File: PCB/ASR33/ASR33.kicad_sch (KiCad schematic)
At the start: 40 parts, among them J2 DC, J3 Power, J4 RUN, J5 Tx, J6 Rx, J7 USB-C-Socket-V, J8 Shelly, Q1 NX7002AK, SW1 SW_Push, U10 ESP32-S3-MINI-1, U2 MD8942, U3 NCR402U, U4 NCR402U, U5 LTV-356T, U7 QR

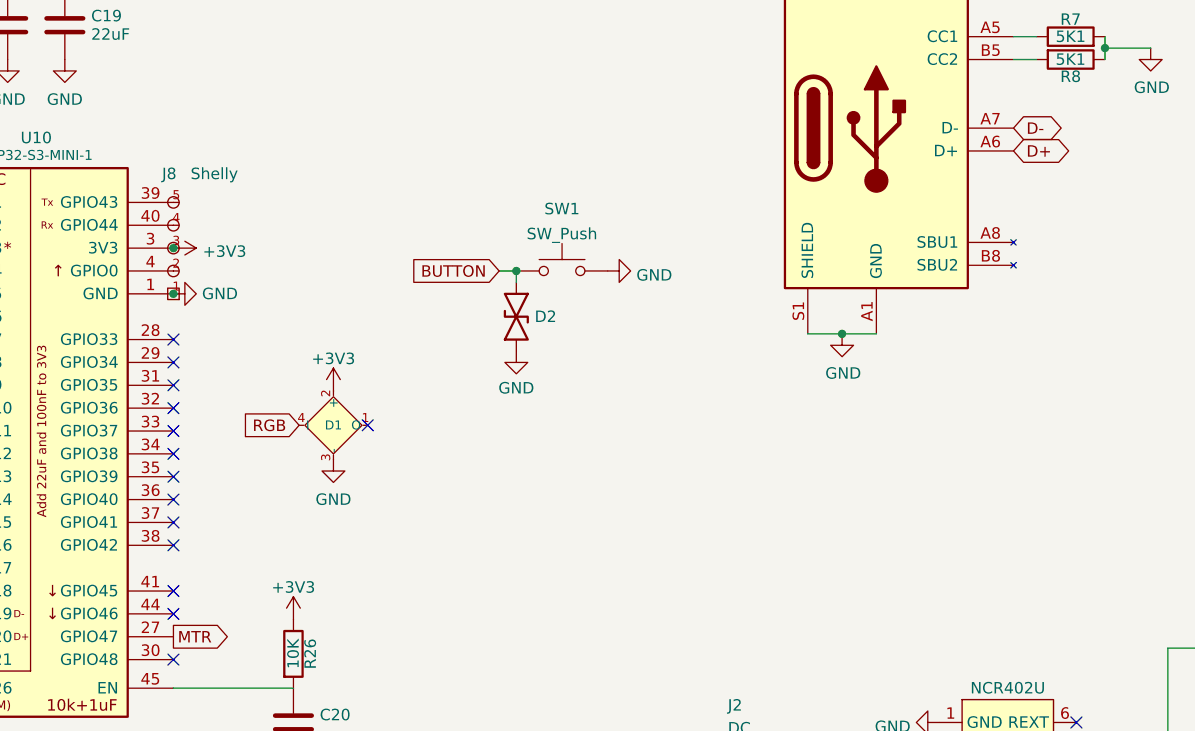
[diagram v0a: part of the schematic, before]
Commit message: Tweaks
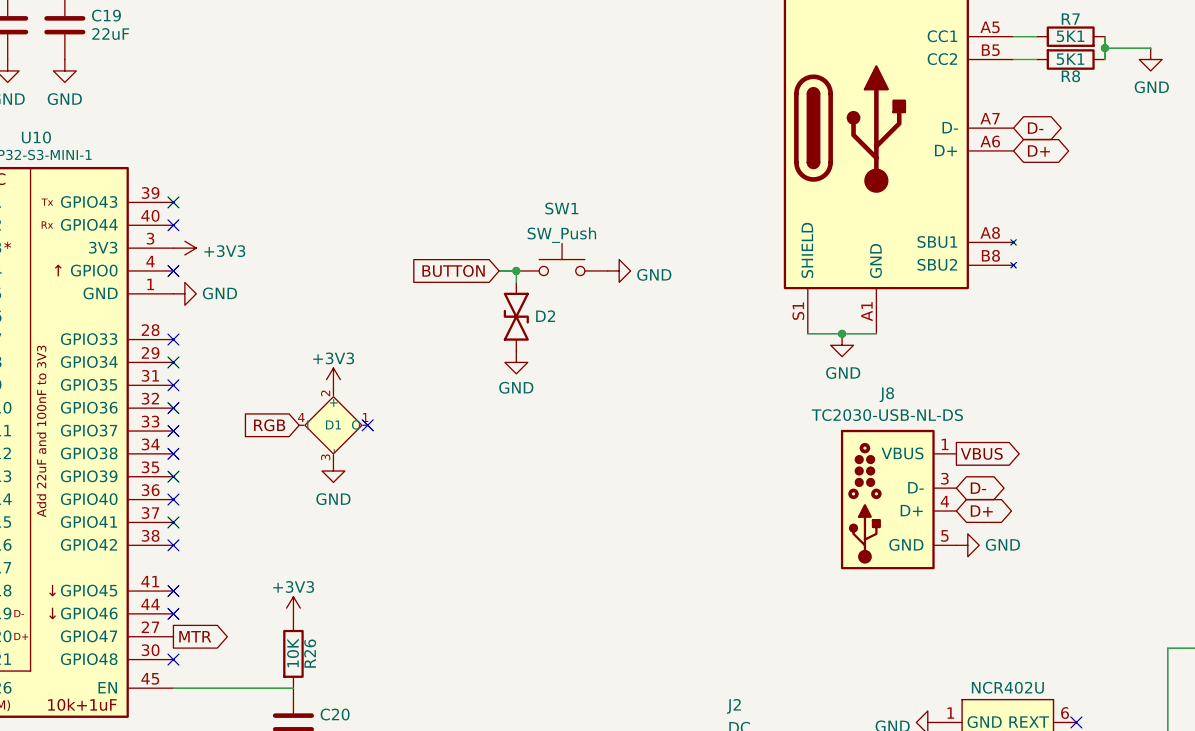
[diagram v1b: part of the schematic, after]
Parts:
- removed J8: Shelly, RevK:Shelly, symbol RevK:Shelly
- added J8: TC2030-USB-NL-DS, RevK:Tag-Connect_TC2030-IDC-NL_2x03_P1.27mm_Vertical, symbol RevK:TC2030-USB-NL
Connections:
- net D+: now also J8.4 (D+)
- net D-: now also J8.3 (D-)
- net GND: now also J8.5 (GND), J8.6 (GND)
- net VBUS: now also J8.1 (VBUS), J8.2 (VBUS)
- no-connect marks 30 -> 33
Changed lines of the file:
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@@
 	)
 	(junction
-		(at 77.47 53.975)
-		(diameter 0)
-		(color 0 0 0 0)
-	)
-	(junction
 		(at 187.96 142.24)
 		(diameter 0)
@@
 	)
 	(junction
-		(at 77.47 59.055)
-		(diameter 0)
-		(color 0 0 0 0)
-	)
-	(junction
 		(at 187.96 111.76)
 		(diameter 0)
@@
 	)
 	(no_connect
+		(at 77.47 48.895)
+	)
+	(no_connect
 		(at 46.99 66.675)
 	)
@@
 	)
 	(no_connect
+		(at 77.47 56.515)
+	)
+	(no_connect
 		(at 46.99 48.895)
 	)
@@
 	)
 	(no_connect
+		(at 77.47 51.435)
+	)
+	(no_connect
 		(at 77.47 81.915)
 	)
@@
 		)
 	)
+	(global_label "D-"
+		(shape bidirectional)
+		(at 164.465 80.645 0)
+		(fields_autoplaced yes)
+		(effects
+			(font
+				(size 1.27 1.27)
+			)
+			(justify left)
+		)
+		(property "Intersheetrefs" "${INTERSHEET_REFS}"
+			(at 170.5909 80.645 0)
+			(effects
+				(font
+					(size 1.27 1.27)
+				)
+				(justify left)
+				(hide yes)
+			)
+		)
+	)
 	(global_label "PWR"
 		(shape input)
@@
 		)
 	)
+	(global_label "VBUS"
+		(shape output)
+		(at 164.465 76.835 0)
+		(fields_autoplaced yes)
+		(effects
+			(font
+				(size 1.27 1.27)
+			)
+			(justify left)
+		)
+		(property "Intersheetrefs" "${INTERSHEET_REFS}"
+			(at 171.6946 76.835 0)
+			(effects
+				(font
+					(size 1.27 1.27)
+				)
+				(justify left)
+				(hide yes)
+			)
+		)
+	)
 	(global_label "DC"
 		(shape input)
@@
 		)
 	)
+	(global_label "D+"
+		(shape bidirectional)
+		(at 164.465 83.185 0)
+		(fields_autoplaced yes)
+		(effects
+			(font
+				(size 1.27 1.27)
+			)
+			(justify left)
+		)
+		(property "Intersheetrefs" "${INTERSHEET_REFS}"
+			(at 170.5909 83.185 0)
+			(effects
+				(font
+					(size 1.27 1.27)
+				)
+				(justify left)
+				(hide yes)
+			)
+		)
+	)
 	(global_label "BUTTON"
 		(shape input)
@@
 	)
 	(symbol
+		(lib_id "RevK:TC2030-USB-NL")
+		(at 156.845 81.915 0)
+		(unit 1)
+		(exclude_from_sim no)
+		(in_bom no)
+		(on_board yes)
+		(dnp no)
+		(fields_autoplaced yes)
+		(property "Reference" "J8"
+			(at 156.845 70.1505 0)
+			(effects
+				(font
+					(size 1.27 1.27)
+				)
+			)
+		)
+		(property "Value" "TC2030-USB-NL-DS"
+			(at 156.845 72.5748 0)
+			(effects
+				(font
+					(size 1.27 1.27)
+				)
+			)
+		)
+		(property "Footprint" "RevK:Tag-Connect_TC2030-IDC-NL_2x03_P1.27mm_Vertical"
+			(at 156.591 91.059 0)
+			(effects
+				(font
+					(size 1.27 1.27)
+				)
+				(hide yes)
+			)
+		)
+		(property "Datasheet" " ~"
+			(at 160.655 83.185 0)
+			(effects
+				(font
+					(size 1.27 1.27)
+				)
+				(hide yes)
+			)
+		)
+		(property "Description" "TC2030-USB-NL"
+			(at 156.845 69.215 0)
+			(effects
+				(font
+					(size 1.27 1.27)
+				)
+				(hide yes)
+			)
+		)
+		(pin "1"
+		)
+		(pin "2"
+		)
+		(pin "3"
+		)
+		(pin "4"
+		)
+		(pin "5"
+		)
+		(pin "6"
+		)
+		(instances
+			(project "ASR33"
+				(path "/46c350bb-7de4-4e81-aafd-4af55e37aab0"
+					(reference "J8")
+					(unit 1)
+				)
+			)
+		)
+	)
+	(symbol
 		(lib_id "RevK:Hidden")
 		(at 256.54 43.18 90)
@@
 	)
 	(symbol
+		(lib_id "power:GND")
+		(at 164.465 86.995 90)
+		(unit 1)
+		(exclude_from_sim no)
+		(in_bom yes)
+		(on_board yes)
+		(dnp no)
+		(fields_autoplaced yes)
+		(property "Reference" "#PWR012"
+			(at 170.815 86.995 0)
+			(effects
+				(font
+					(size 1.27 1.27)
+				)
+				(hide yes)
+			)
+		)
+		(property "Value" "GND"
+			(at 167.64 86.995 90)
+			(effects
+				(font
+					(size 1.27 1.27)
+				)
+				(justify right)
+			)
+		)
+		(property "Footprint" ""
+			(at 164.465 86.995 0)
+			(effects
+				(font
+					(size 1.27 1.27)
+				)
+				(hide yes)
+			)
+		)
+		(property "Datasheet" ""
+			(at 164.465 86.995 0)
+			(effects
+				(font
+					(size 1.27 1.27)
+				)
+				(hide yes)
+			)
+		)
+		(property "Description" "Power symbol creates a global label with name \"GND\" , ground"
+			(at 164.465 86.995 0)
+			(effects
+				(font
+					(size 1.27 1.27)
+				)
+				(hide yes)
+			)
+		)
+		(pin "1"
+		)
+		(instances
+			(project "ASR33"
+				(path "/46c350bb-7de4-4e81-aafd-4af55e37aab0"
+					(reference "#PWR012")
+					(unit 1)
+				)
+			)
+		)
+	)
+	(symbol
 		(lib_id "RevK:VCUT")
 		(at 263.525 173.99 90)
@@
 					(unit 1)
 				)
-			)
-		)
-	)
-	(symbol
-		(lib_id "RevK:Shelly")
-		(at 77.47 53.975 0)
-		(unit 1)
-		(exclude_from_sim no)
-		(in_bom no)
-		(on_board yes)
-		(dnp no)
-		(property "Reference" "J8"
-			(at 76.2 45.72 0)
-			(effects
-				(font
-					(size 1.27 1.27)
-				)
-				(justify left)
-			)
-		)
-		(property "Value" "Shelly"
-			(at 79.375 45.72 0)
-			(effects
-				(font
-					(size 1.27 1.27)
-				)
-				(justify left)
-			)
-		)
-		(property "Footprint" "RevK:Shelly"
-			(at 80.01 62.23 0)
-			(effects
-				(font
-					(size 1.27 1.27)
-				)
-				(hide yes)
-			)
-		)
-		(property "Datasheet" ""
-			(at 80.01 62.23 0)
-			(effects
-				(font
-					(size 1.27 1.27)
-				)
-				(hide yes)
-			)
-		)
-		(property "Description" ""
-			(at 77.47 53.975 0)
-			(effects
-				(font
-					(size 1.27 1.27)
-				)
-				(hide yes)
-			)
-		)
-		(pin "1"
-		)
-		(pin "2"
-		)
-		(pin "3"
-		)
-		(pin "4"
-		)
-		(pin "5"
-		)
-		(instances
-			(project "Access"
-				(path "/2a267270-6585-45e3-a633-b53049f10066"
-					(reference "J8")
-					(unit 1)
-				)
-			)
-			(project "USBA"
-				(path "/2d210a96-f81f-42a9-8bf4-1b43c11086f3"
-					(reference "J2")
-					(unit 1)
-				)
-			)
-			(project "ASR33"
-				(path "/46c350bb-7de4-4e81-aafd-4af55e37aab0"
-					(reference "J8")
-					(unit 1)
-				)
